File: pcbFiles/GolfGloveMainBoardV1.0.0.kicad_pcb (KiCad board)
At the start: 4 copper layers, 40 x 55.3 mm, 129 parts, among them J1 USB_C_Receptacle, J11 Conn_01x16_Male, J12 HOST_WAKE, J13 TP4, J14 Conn_01x02, J15 Conn_01x02, J16 Conn_01x02, J17 Conn_01x02, J2 Conn_01x06, J3 USB_C_Receptacle, J6 Screw_Terminal_01x02, J7 Conn_01x02, J8 Conn_01x02, J9 Conn_01x02, SW1 SW_SPDT, SW2 SW_Push, U1 MCP73831T-2ACI/OT, U2 XC6119N16A7R-G, U3 LSM9DS1TR, U4 CYW20719B1KUMLG, U5 LSM9DS1TR, U7 TPS63001DRCT, Y1 Crystal, Y2 Crystal_GND23

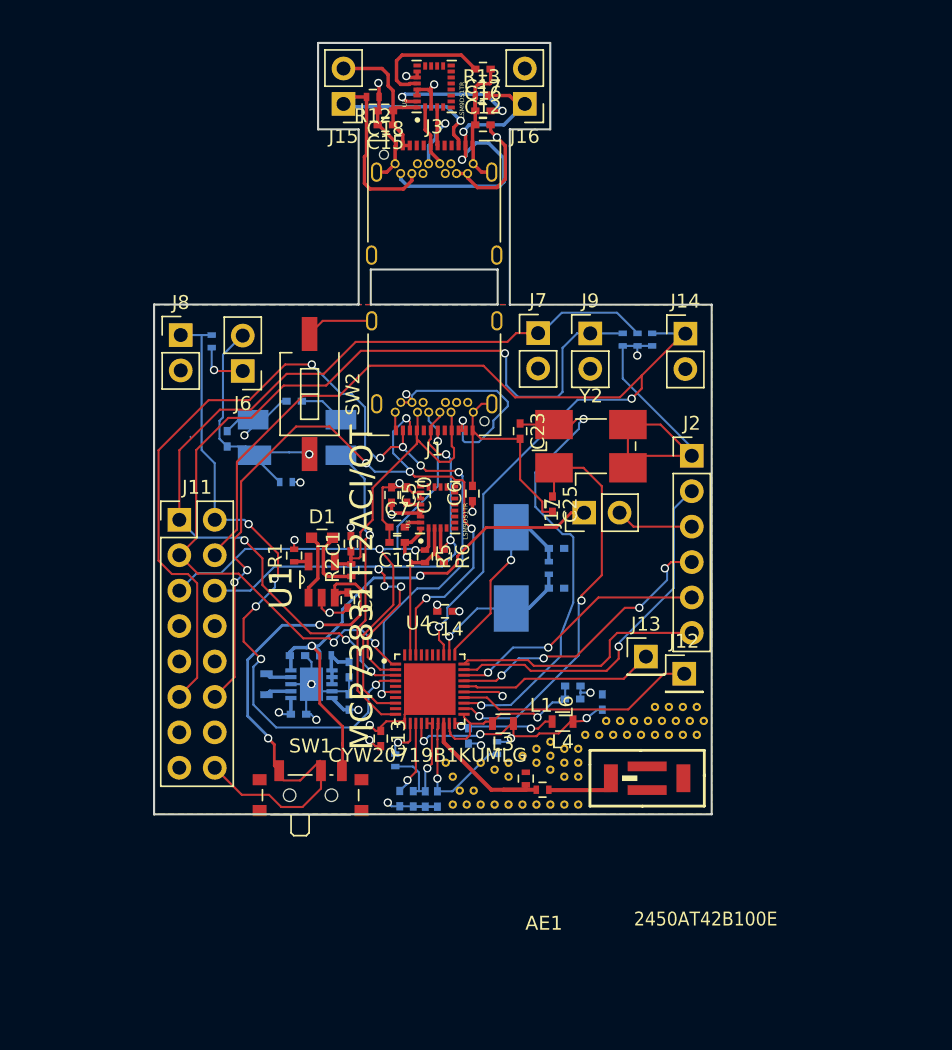
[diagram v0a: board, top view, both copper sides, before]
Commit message: Update Docs
@willcarroll7
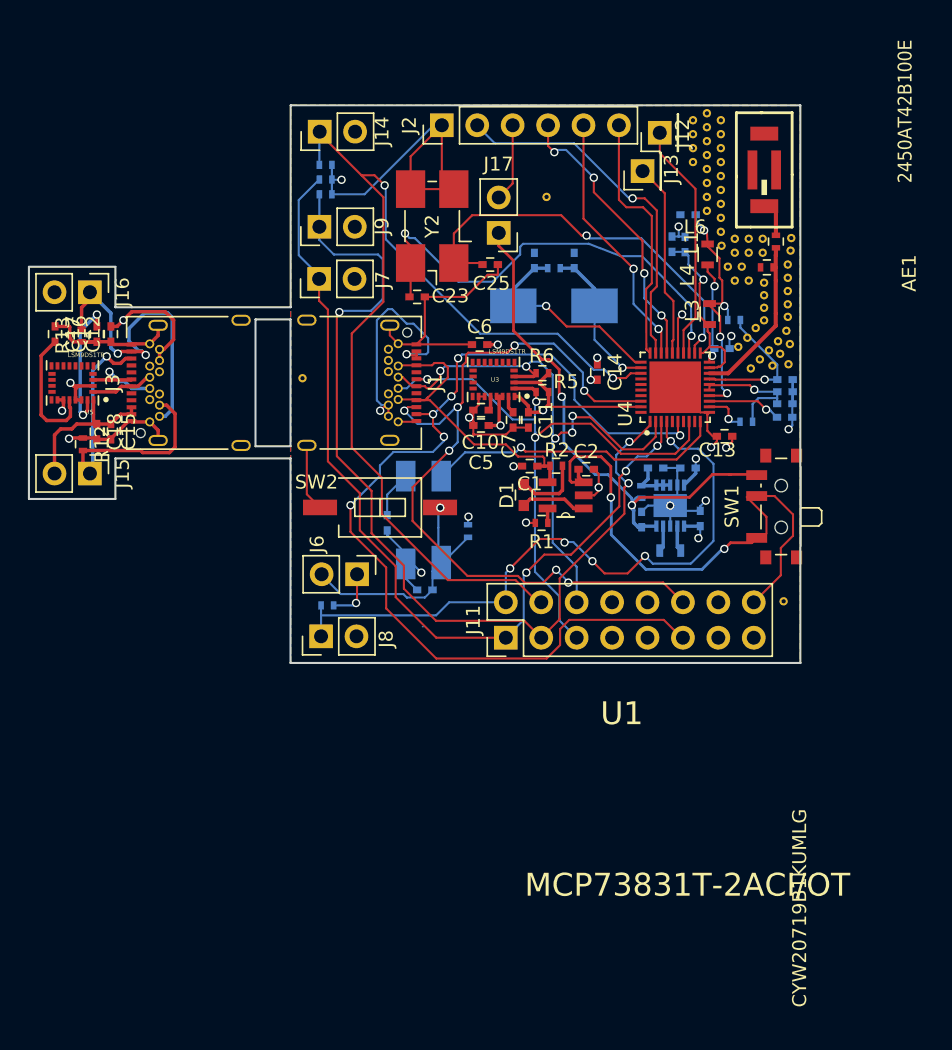
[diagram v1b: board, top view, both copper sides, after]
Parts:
- removed the REF** at (126.0, 158.5)
- removed the REF** at (124.5, 160.5)
- added REF**: VIA-0.6mm, VIA-0.6mm, F.Cu at (148.3, 120.9)
- added REF**: VIA-0.6mm, VIA-0.6mm, F.Cu at (147.3, 128.3)
- added REF**: VIA-0.6mm, VIA-0.6mm, F.Cu at (146.9, 130.0)
- added REF**: VIA-0.6mm, VIA-0.6mm, F.Cu at (143.3, 121.4)
- added REF**: VIA-0.6mm, VIA-0.6mm, F.Cu at (146.3, 124.1)
- added REF**: VIA-0.6mm, VIA-0.6mm, F.Cu at (144.5, 128.7)
- added REF**: VIA-0.6mm, VIA-0.6mm, F.Cu at (109.7, 131.9)
- added REF**: VIA-0.6mm, VIA-0.6mm, F.Cu at (144.2, 147.9)
- added REF**: VIA-0.6mm, VIA-0.6mm, F.Cu at (127.2, 118.9)
- moved AE1 44.4 mm to (146.3, 116.0), turned to 90 degrees
- moved REF** 44.1 mm to (143.2, 112.4), turned to 90 degrees
- moved REF** 43.6 mm to (142.2, 111.9), turned to 90 degrees
- moved REF** 43.2 mm to (143.2, 113.4), turned to 90 degrees
- moved L1 42.7 mm to (147.2, 121.1), turned to 90 degrees
- moved REF** 42.6 mm to (142.2, 112.9), turned to 90 degrees
- moved REF** 42.5 mm to (148.2, 121.8), turned to 90 degrees
- moved REF** 42.2 mm to (143.2, 114.4), turned to 90 degrees
- moved REF** 42.1 mm to (141.2, 112.4), turned to 90 degrees
- moved REF** 41.9 mm to (148.0, 122.8), turned to 90 degrees
- moved REF** 41.6 mm to (142.2, 113.9), turned to 90 degrees
- moved REF** 41.4 mm to (148.0, 123.7), turned to 90 degrees
- moved REF** 41.3 mm to (143.2, 115.4), turned to 90 degrees
- moved REF** 41.1 mm to (141.2, 113.4), turned to 90 degrees
- moved REF** 40.8 mm to (146.2, 120.9), turned to 90 degrees
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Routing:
- net 3.3v: track 218.0 -> 330.0 mm
- net Net-(AE1-Pad1): track 4.35 -> 2.84 mm
- net Net-(L1-Pad1): track 11.3 -> 12.0 mm
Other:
- board size 40 x 55.3 mm -> 55.3 x 40 mm
- net class 3v added: clearance 0.2, trace_width 0.3, via_dia 0.45, via_drill 0.2
- board text added: "Golf Glove"
- board text added: "LEC"
- board text added: "REV1.0"
